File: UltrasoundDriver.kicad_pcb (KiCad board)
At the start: 2 copper layers, 137.3 x 46.2 mm, 52 parts, among them J1 Conn_01x05_Female, J2 Conn_01x05_Female, Q1 SS8050-G, Q2 S8550, U1 MC33079, U2 L7815, U3 L7915, U4 MC33079

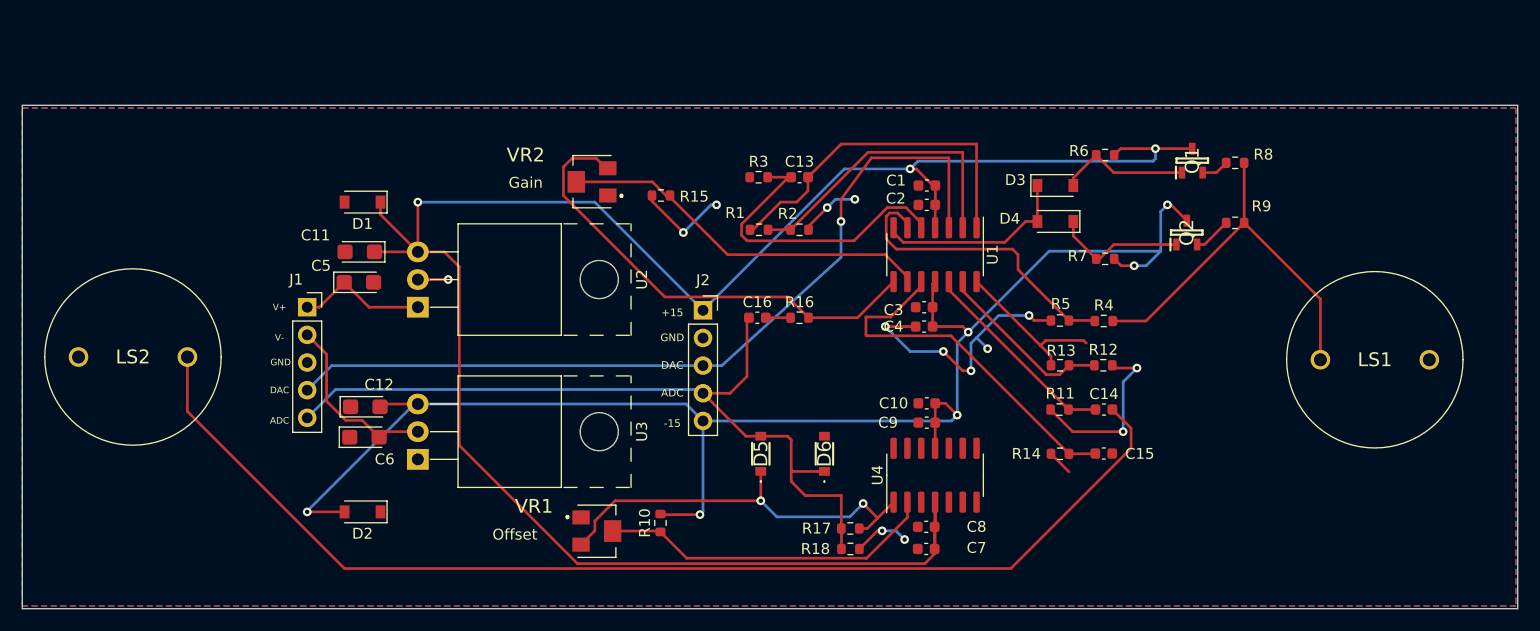
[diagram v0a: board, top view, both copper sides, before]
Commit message: updated and sent to Justin
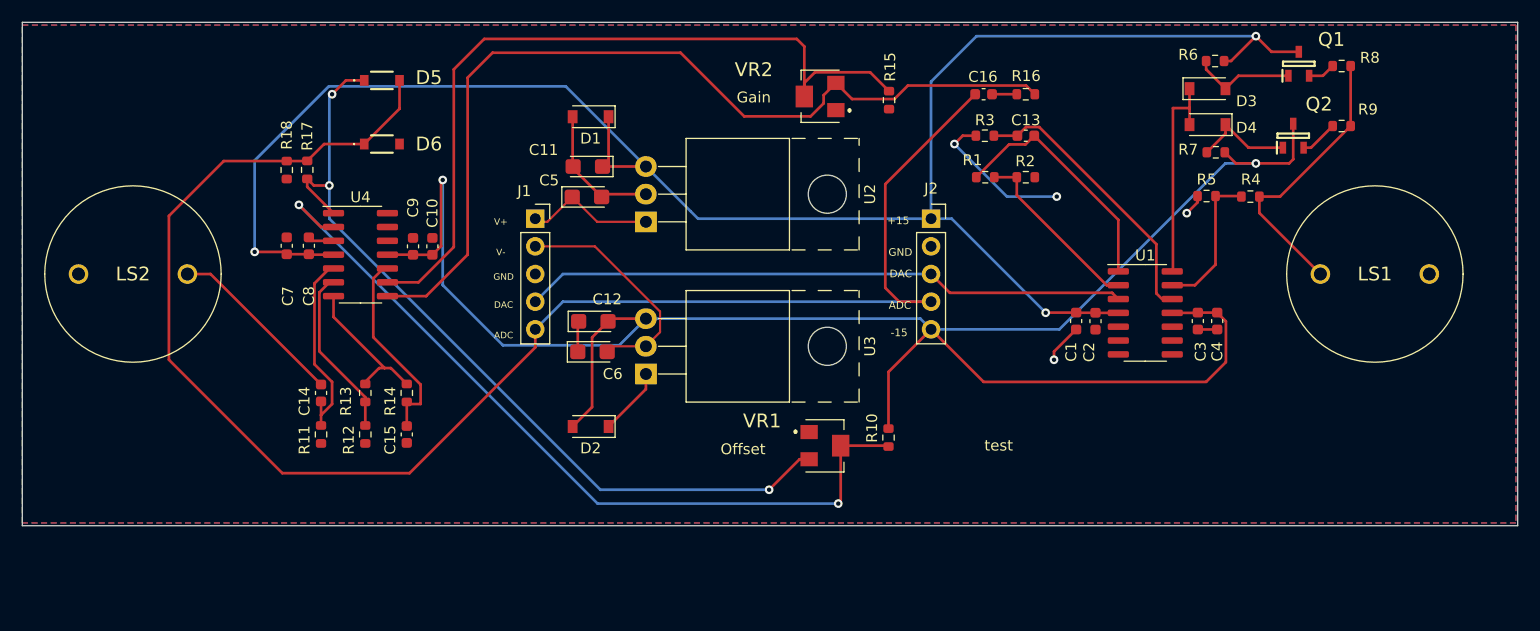
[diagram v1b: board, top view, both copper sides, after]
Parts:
- moved C14 71.9 mm to (126.5, 74.4), turned to 90 degrees
- moved R12 68.1 mm to (130.6, 78.2), turned to -90 degrees
- moved R11 67.9 mm to (126.5, 78.2), turned to -90 degrees
- moved C7 65.0 mm to (123.3, 60.9), turned to 90 degrees
- moved C15 64.0 mm to (134.4, 78.2), turned to 90 degrees
- moved R13 63.8 mm to (130.6, 74.4), turned to 90 degrees
- moved R18 62.4 mm to (123.3, 53.9), turned to 90 degrees
- moved C8 62.3 mm to (125.4, 60.9), turned to 90 degrees
- moved R14 60.2 mm to (134.4, 74.4), turned to -90 degrees
- moved R17 59.8 mm to (125.2, 53.9), turned to -90 degrees
- moved U4 56.5 mm to (130.1, 61.7), turned to 0 degrees
- moved C9 49.9 mm to (134.9, 61.0), turned to 90 degrees
- moved D6 49.6 mm to (132.1, 51.6), turned to 0 degrees
- moved D5 48.9 mm to (132.1, 45.7), turned to 0 degrees
- moved C10 47.6 mm to (136.7, 61.0), turned to 90 degrees
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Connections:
- D3 pad 1: Net-(U1-Pad7) -> Net-(D3-Pad1)
- D4 pad 2: Net-(U1-Pad7) -> Net-(D3-Pad1)
- U1 pad 10: Net-(C15-Pad2) -> (no net)
- U1 pad 12: Net-(C14-Pad1) -> Net-(C13-Pad1)
- U1 pad 13: Net-(R12-Pad1) -> Net-(R4-Pad2)
- U1 pad 14: Net-(R13-Pad2) -> Net-(D3-Pad1)
- U1 pad 5: Net-(C13-Pad1) -> (no net)
- U1 pad 6: Net-(R4-Pad2) -> (no net)
- U1 pad 7: Net-(U1-Pad7) -> (no net)
- U1 pad 8: Net-(R16-Pad2) -> (no net)
- U1 pad 9: Net-(R15-Pad1) -> (no net)
- U4 pad 10: (no net) -> Net-(C15-Pad2)
- U4 pad 5: (no net) -> Net-(C14-Pad1)
- U4 pad 6: (no net) -> Net-(R12-Pad1)
- U4 pad 7: (no net) -> Net-(R13-Pad2)
- U4 pad 8: (no net) -> Net-(R16-Pad2)
- U4 pad 9: (no net) -> Net-(R15-Pad1)
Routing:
- net Net-(C14-Pad2): track 106.5 -> 16.5 mm
- net sigOut: track 74.9 -> 149.9 mm
- net Net-(R10-Pad1): track 31.1 -> 74.8 mm, vias 0 -> 2
- net -15V: track 139.2 -> 180.0 mm, vias 6 -> 2
- net Net-(R16-Pad2): track 43.7 -> 83.8 mm
- net 3.3V: track 38.0 -> 77.0 mm, vias 2 -> 3
- net Net-(R15-Pad1): track 34.5 -> 72.1 mm
- net sigIn: track 77.4 -> 55.5 mm, vias 1 -> 0
- net Net-(D3-Pad1): track 0.00 -> 19.9 mm
- net GND: track 63.4 -> 45.2 mm, vias 14 -> 4
- net Net-(U1-Pad7): track 18.1 -> 0.00 mm
- net +15V: track 185.7 -> 167.8 mm
- net Net-(C15-Pad2): track 33.9 -> 18.6 mm
- net Net-(R4-Pad2): track 28.1 -> 13.5 mm
- net Net-(R1-Pad2): track 27.8 -> 16.5 mm
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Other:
- board text added: "test"
